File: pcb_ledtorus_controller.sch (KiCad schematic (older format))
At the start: 27 parts, among them P7 CONN_4X2, P8 CONN_9, U1 TM4C1232XXPM, U3 KNUSB, X1 NX5032GA-16MHz

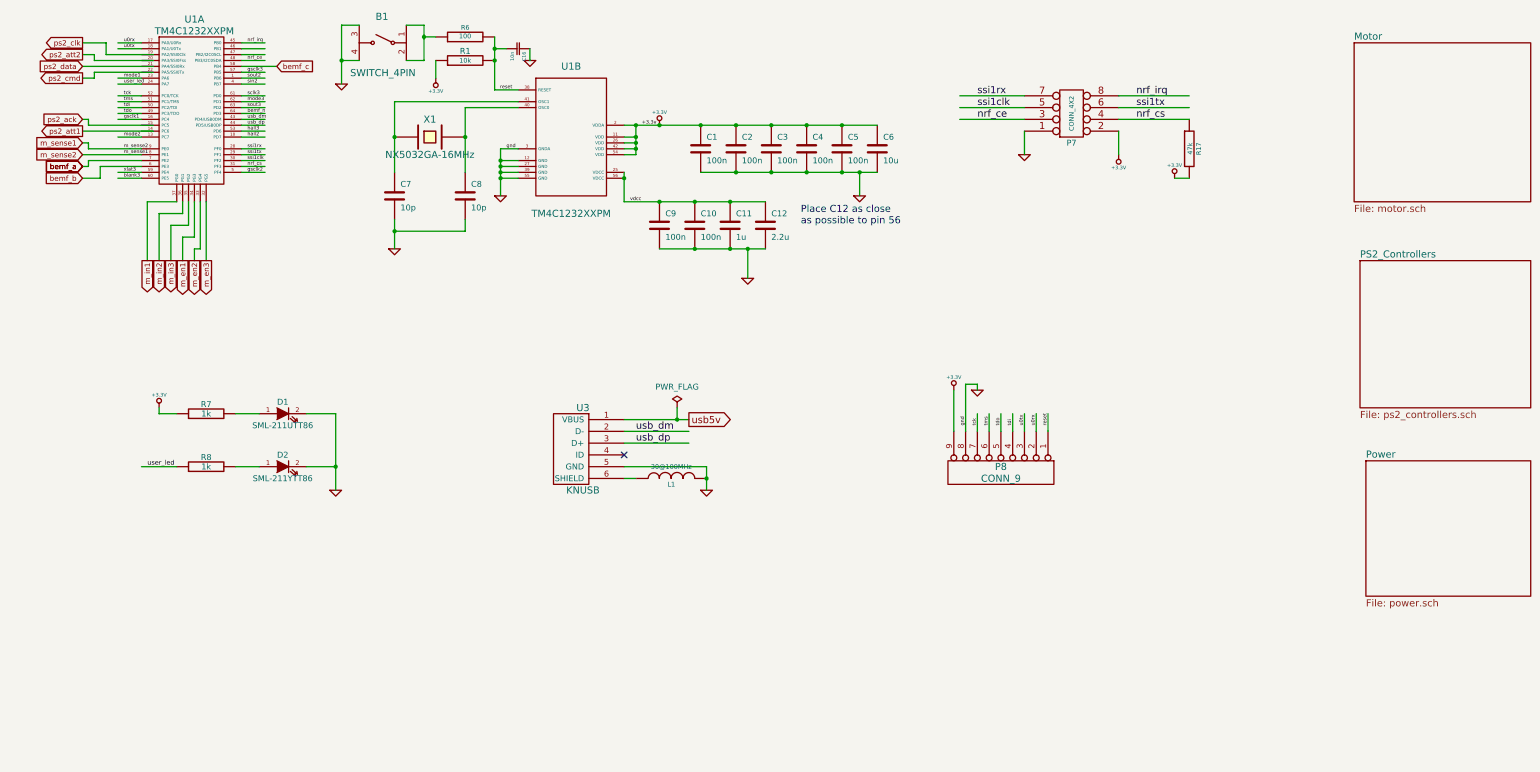
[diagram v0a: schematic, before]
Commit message: Passing ERC
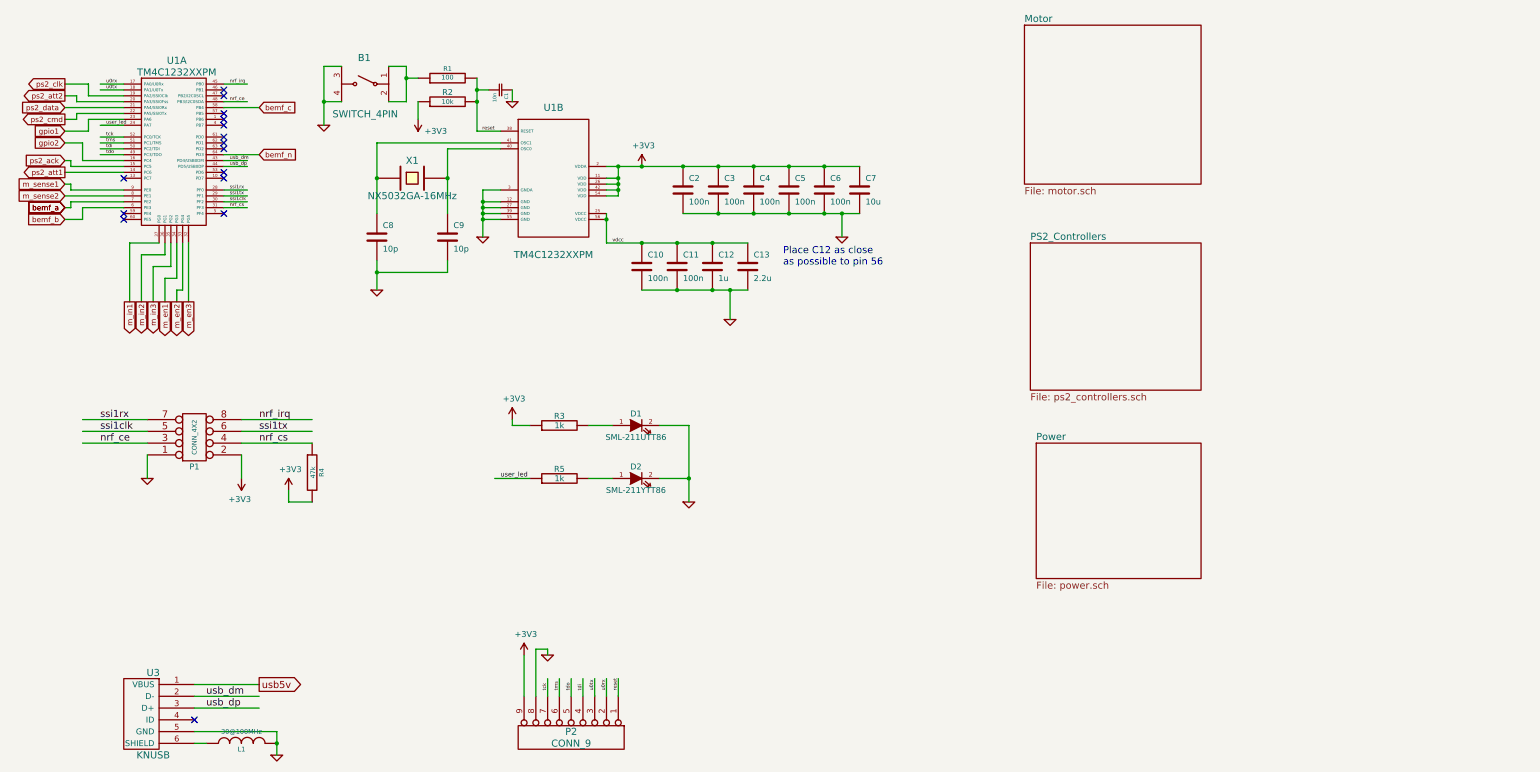
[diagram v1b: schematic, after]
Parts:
- renumbered C16 to C1, C9 to C10, C10 to C11, C11 to C12, C12 to C13, C1 to C2, C2 to C3, C3 to C4, C4 to C5, C5 to C6, C6 to C7, C7 to C8, C8 to C9, P7 to P1, P8 to P2, R6 to R1, R1 to R2, R7 to R3, R17 to R4, R8 to R5
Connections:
- net labels added: +3V3, gpio1, gpio2
- net labels removed: +3.3V, +3.3v, blank3, gnd, gsclk1, gsclk2, gsclk3, hall2, hall3, mode1, mode2, mode3, sclk3, sin2, sout2, sout3, xlat3
- wire segments 144 -> 134
- no-connect marks 1 -> 15
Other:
- moved on the sheet: B1, C1, C10, C11, C12, C13, C2, C3, C4, C5, C6, C7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

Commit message: Starting on netlist
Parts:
- B1: footprint (none) -> knielsenlib:SWITCH_FSMJSMA
- C1, C12, C13, C7, C8, C9: footprint (none) -> Capacitors_SMD:C_0805
- C10, C11, C2, C3, C4, C5, C6: footprint (none) -> Capacitors_SMD:C_0603
- D1, D2: footprint (none) -> LEDs:LED_0805
- L1: footprint (none) -> Inductors_SMD:L_0603
- P1: footprint (none) -> Pin_Headers:Pin_Header_Straight_2x04_Pitch1.27mm
- P2: footprint (none) -> Pin_Headers:Pin_Header_Straight_1x09_Pitch1.27mm
- R1, R2, R3, R4, R5: footprint (none) -> Resistors_SMD:R_0805
- U1: footprint (none) -> knielsenlib:LQFP_64
- U3: footprint (none) -> knielsenlib:10103594-0001LF
- X1: footprint (none) -> knielsenlib:NX5032GA
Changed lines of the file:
@@
 LIBS:w_device
 LIBS:pcb_ledtorus_controller-cache
-LIBS:tiva_pcb1-cache
 EELAYER 26 0
 EELAYER END
@@
 F 0 "R2" V 4630 1550 50  0000 C CNN
 F 1 "10k" V 4550 1550 40  0000 C CNN
-F 2 "" H 4550 1550 60  0001 C CNN
+F 2 "Resistors_SMD:R_0805" H 4550 1550 60  0001 C CNN
 F 3 "" H 4550 1550 60  0001 C CNN
 	1    4550 1550
@@
 F 0 "C7" H 8100 2400 50  0000 L CNN
 F 1 "10u" H 8100 2200 50  0000 L CNN
-F 2 "" H 8050 2300 60  0001 C CNN
+F 2 "Capacitors_SMD:C_0805" H 8050 2300 60  0001 C CNN
 F 3 "" H 8050 2300 60  0001 C CNN
 	1    8050 2300
@@
 F 0 "C6" H 7800 2400 50  0000 L CNN
 F 1 "100n" H 7800 2200 50  0000 L CNN
-F 2 "" H 7750 2300 60  0001 C CNN
+F 2 "Capacitors_SMD:C_0603" H 7750 2300 60  0001 C CNN
 F 3 "" H 7750 2300 60  0001 C CNN
 	1    7750 2300
@@
 F 0 "C2" H 6600 2400 50  0000 L CNN
 F 1 "100n" H 6600 2200 50  0000 L CNN
-F 2 "" H 6550 2300 60  0001 C CNN
+F 2 "Capacitors_SMD:C_0603" H 6550 2300 60  0001 C CNN
 F 3 "" H 6550 2300 60  0001 C CNN
 	1    6550 2300
@@
 F 0 "C3" H 6900 2400 50  0000 L CNN
 F 1 "100n" H 6900 2200 50  0000 L CNN
-F 2 "" H 6850 2300 60  0001 C CNN
+F 2 "Capacitors_SMD:C_0603" H 6850 2300 60  0001 C CNN
 F 3 "" H 6850 2300 60  0001 C CNN
 	1    6850 2300
@@
 F 0 "C4" H 7200 2400 50  0000 L CNN
 F 1 "100n" H 7200 2200 50  0000 L CNN
-F 2 "" H 7150 2300 60  0001 C CNN
+F 2 "Capacitors_SMD:C_0603" H 7150 2300 60  0001 C CNN
 F 3 "" H 7150 2300 60  0001 C CNN
 	1    7150 2300
@@
 F 0 "C5" H 7500 2400 50  0000 L CNN
 F 1 "100n" H 7500 2200 50  0000 L CNN
-F 2 "" H 7450 2300 60  0001 C CNN
+F 2 "Capacitors_SMD:C_0603" H 7450 2300 60  0001 C CNN
 F 3 "" H 7450 2300 60  0001 C CNN
 	1    7450 2300
@@
 F 0 "C13" H 7150 3050 50  0000 L CNN
 F 1 "2.2u" H 7150 2850 50  0000 L CNN
-F 2 "" H 7100 2950 60  0001 C CNN
+F 2 "Capacitors_SMD:C_0805" H 7100 2950 60  0001 C CNN
 F 3 "" H 7100 2950 60  0001 C CNN
 	1    7100 2950
@@
 F 0 "C12" H 6850 3050 50  0000 L CNN
 F 1 "1u" H 6850 2850 50  0000 L CNN
-F 2 "" H 6800 2950 60  0001 C CNN
+F 2 "Capacitors_SMD:C_0805" H 6800 2950 60  0001 C CNN
 F 3 "" H 6800 2950 60  0001 C CNN
 	1    6800 2950
@@
 F 0 "C11" H 6550 3050 50  0000 L CNN
 F 1 "100n" H 6550 2850 50  0000 L CNN
-F 2 "" H 6500 2950 60  0001 C CNN
+F 2 "Capacitors_SMD:C_0603" H 6500 2950 60  0001 C CNN
 F 3 "" H 6500 2950 60  0001 C CNN
 	1    6500 2950
@@
 F 0 "C10" H 6250 3050 50  0000 L CNN
 F 1 "100n" H 6250 2850 50  0000 L CNN
-F 2 "" H 6200 2950 60  0001 C CNN
+F 2 "Capacitors_SMD:C_0603" H 6200 2950 60  0001 C CNN
 F 3 "" H 6200 2950 60  0001 C CNN
 	1    6200 2950
@@
 F 0 "C9" H 4600 2800 50  0000 L CNN
 F 1 "10p" H 4600 2600 50  0000 L CNN
-F 2 "" H 4550 2700 60  0001 C CNN
+F 2 "Capacitors_SMD:C_0805" H 4550 2700 60  0001 C CNN
 F 3 "" H 4550 2700 60  0001 C CNN
 	1    4550 2700
@@
 F 0 "C8" H 4000 2800 50  0000 L CNN
 F 1 "10p" H 4000 2600 50  0000 L CNN
-F 2 "" H 3950 2700 60  0001 C CNN
+F 2 "Capacitors_SMD:C_0805" H 3950 2700 60  0001 C CNN
 F 3 "" H 3950 2700 60  0001 C CNN
 	1    3950 2700
@@
 F 0 "X1" H 4250 2350 60  0000 C CNN
 F 1 "NX5032GA-16MHz" H 4250 2050 60  0000 C CNN
-F 2 "" H 4250 2200 60  0001 C CNN
+F 2 "knielsenlib:NX5032GA" H 4250 2200 60  0001 C CNN
 F 3 "" H 4250 2200 60  0001 C CNN
 	1    4250 2200
@@
 F 0 "U1" H 5450 2700 60  0000 C CNN
 F 1 "TM4C1232XXPM" H 5450 1450 60  0000 C CNN
-F 2 "" H 5450 2150 60  0001 C CNN
+F 2 "knielsenlib:LQFP_64" H 5450 2150 60  0001 C CNN
 F 3 "" H 5450 2150 60  0001 C CNN
 	2    5450 2150
@@
 F 0 "U1" H 2250 2800 60  0000 C CNN
 F 1 "TM4C1232XXPM" H 2250 2700 60  0000 C CNN
-F 2 "" H 2250 2000 60  0000 C CNN
+F 2 "knielsenlib:LQFP_64" H 2250 2000 60  0001 C CNN
 F 3 "" H 2250 2000 60  0000 C CNN
 	1    2250 2000
@@
 F 0 "U3" H 2050 6400 60  0000 C CNN
 F 1 "KNUSB" H 2050 5700 60  0000 C CNN
-F 2 "" H 2050 6400 60  0000 C CNN
+F 2 "knielsenlib:10103594-0001LF" H 2050 6400 60  0001 C CNN
 F 3 "" H 2050 6400 60  0000 C CNN
 	1    2050 6400
@@
 F 0 "L1" V 2750 7000 40  0000 C CNN
 F 1 "30@100MHz" V 2900 7000 40  0000 C CNN
-F 2 "" H 2800 7000 60  0000 C CNN
+F 2 "Inductors_SMD:L_0603" H 2800 7000 60  0001 C CNN
 F 3 "" H 2800 7000 60  0000 C CNN
 	1    2800 7000
@@
 F 0 "B1" H 3857 1623 60  0000 C CNN
 F 1 "SWITCH_4PIN" H 3849 1145 60  0000 C CNN
-F 2 "" H 3850 1400 60  0000 C CNN
+F 2 "knielsenlib:SWITCH_FSMJSMA" H 3850 1400 60  0001 C CNN
 F 3 "" H 3850 1400 60  0000 C CNN
 	1    3850 1400
@@
 F 0 "R1" V 4630 1350 40  0000 C CNN
 F 1 "100" V 4557 1351 40  0000 C CNN
-F 2 "" V 4480 1350 30  0000 C CNN
+F 2 "Resistors_SMD:R_0805" V 4480 1350 30  0001 C CNN
 F 3 "" H 4550 1350 30  0000 C CNN
 	1    4550 1350
@@
 F 0 "C1" H 5025 1500 30  0000 L CNN
 F 1 "10n" H 5025 1400 30  0000 L CNN
-F 2 "" H 5000 1450 60  0000 C CNN
+F 2 "Capacitors_SMD:C_0805" H 5000 1450 60  0001 C CNN
 F 3 "" H 5000 1450 60  0000 C CNN
 	1    5000 1450
@@
 F 0 "R5" V 5580 4750 50  0000 C CNN
 F 1 "1k" V 5500 4750 50  0000 C CNN
-F 2 "" H 5500 4750 60  0001 C CNN
+F 2 "Resistors_SMD:R_0805" H 5500 4750 60  0001 C CNN
 F 3 "" H 5500 4750 60  0001 C CNN
 	1    5500 4750
@@
 F 0 "R3" V 5580 4300 50  0000 C CNN
 F 1 "1k" V 5500 4300 50  0000 C CNN
-F 2 "" H 5500 4300 60  0001 C CNN
+F 2 "Resistors_SMD:R_0805" H 5500 4300 60  0001 C CNN
 F 3 "" H 5500 4300 60  0001 C CNN
 	1    5500 4300
@@
 F 0 "D2" H 6150 4850 50  0000 C CNN
 F 1 "SML-211YTT86" H 6150 4650 50  0000 C CNN
-F 2 "" H 6150 4750 60  0001 C CNN
+F 2 "LEDs:LED_0805" H 6150 4750 60  0001 C CNN
 F 3 "" H 6150 4750 60  0001 C CNN
 	1    6150 4750
@@
 F 0 "D1" H 6150 4400 50  0000 C CNN
 F 1 "SML-211UTT86" H 6150 4200 50  0000 C CNN
-F 2 "" H 6150 4300 60  0001 C CNN
+F 2 "LEDs:LED_0805" H 6150 4300 60  0001 C CNN
 F 3 "" H 6150 4300 60  0001 C CNN
 	1    6150 4300
@@
 F 0 "P1" H 2400 4650 50  0000 C CNN
 F 1 "CONN_4X2" V 2400 4400 40  0000 C CNN
-F 2 "" H 2400 4400 60  0000 C CNN
+F 2 "Pin_Headers:Pin_Header_Straight_2x04_Pitch1.27mm" H 2400 4400 60  0001 C CNN
 F 3 "" H 2400 4400 60  0000 C CNN
 	1    2400 4400
@@
 F 0 "P2" V 5550 6950 60  0000 C CNN
 F 1 "CONN_9" V 5650 6950 60  0000 C CNN
-F 2 "" H 5600 6950 60  0000 C CNN
+F 2 "Pin_Headers:Pin_Header_Straight_1x09_Pitch1.27mm" H 5600 6950 60  0001 C CNN
 F 3 "" H 5600 6950 60  0000 C CNN
 	1    5600 6950
@@
 F 0 "R4" V 3480 4700 40  0000 C CNN
 F 1 "47k" V 3407 4701 40  0000 C CNN
-F 2 "" V 3330 4700 30  0000 C CNN
+F 2 "Resistors_SMD:R_0805" V 3330 4700 30  0001 C CNN
 F 3 "" H 3400 4700 30  0000 C CNN
 	1    3400 4700

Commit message: Starting on netlist
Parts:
- P1: footprint Pin_Headers:Pin_Header_Straight_2x04_Pitch1.27mm -> Pin_Headers:Pin_Header_Straight_2x04_Pitch2.54mm
- P2: footprint Pin_Headers:Pin_Header_Straight_1x09_Pitch1.27mm -> Pin_Headers:Pin_Header_Straight_1x09_Pitch2.54mm
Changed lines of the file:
@@
 LIBS:contrib
 LIBS:valves
-LIBS:w_analog
-LIBS:w_device
 LIBS:pcb_ledtorus_controller-cache
 EELAYER 26 0
@@
 F 0 "P1" H 2400 4650 50  0000 C CNN
 F 1 "CONN_4X2" V 2400 4400 40  0000 C CNN
-F 2 "Pin_Headers:Pin_Header_Straight_2x04_Pitch1.27mm" H 2400 4400 60  0001 C CNN
+F 2 "Pin_Headers:Pin_Header_Straight_2x04_Pitch2.54mm" H 2400 4400 60  0001 C CNN
 F 3 "" H 2400 4400 60  0000 C CNN
 	1    2400 4400
@@
 F 0 "P2" V 5550 6950 60  0000 C CNN
 F 1 "CONN_9" V 5650 6950 60  0000 C CNN
-F 2 "Pin_Headers:Pin_Header_Straight_1x09_Pitch1.27mm" H 5600 6950 60  0001 C CNN
+F 2 "Pin_Headers:Pin_Header_Straight_1x09_Pitch2.54mm" H 5600 6950 60  0001 C CNN
 F 3 "" H 5600 6950 60  0000 C CNN
 	1    5600 6950

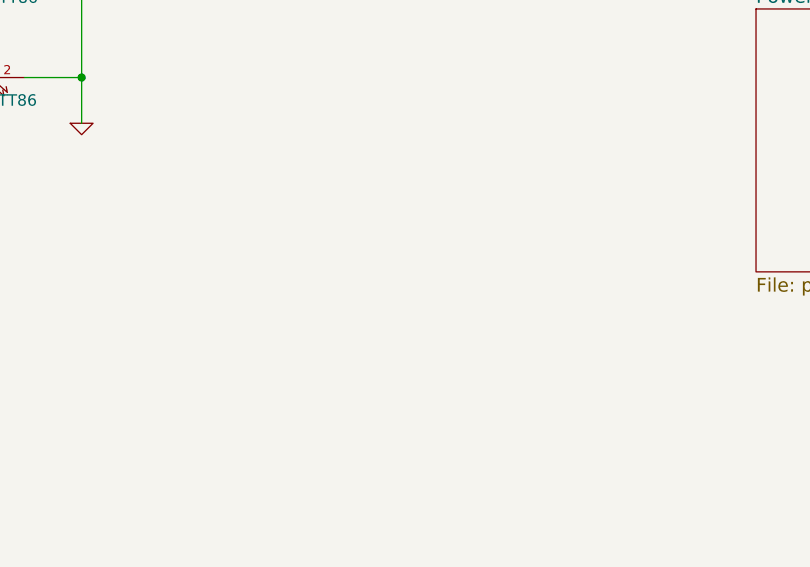
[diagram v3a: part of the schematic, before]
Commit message: Work on layout
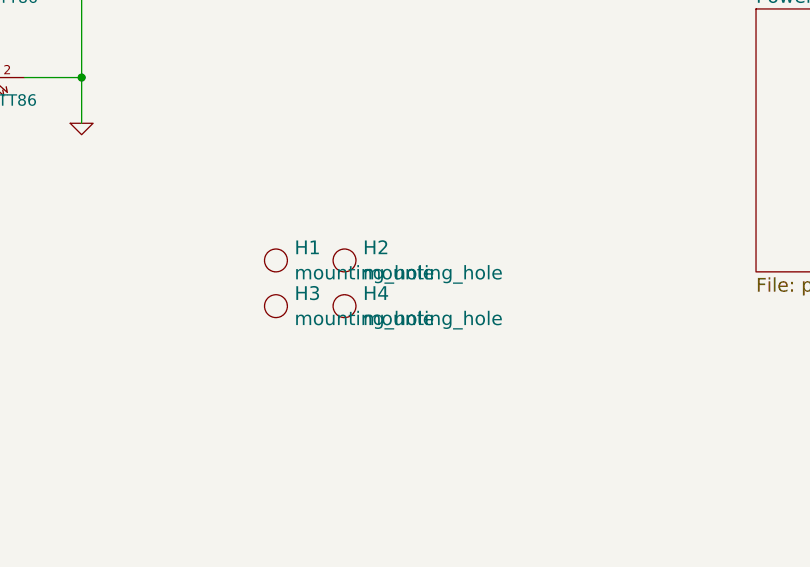
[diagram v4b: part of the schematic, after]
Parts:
- added H1, H2, H3, H4: mounting_hole, Mounting_Holes:MountingHole_4.3mm_M4, symbol mounting_hole
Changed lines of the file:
@@
 	-1   0    0    1
 $EndComp
+$Comp
+L mounting_hole H1
+U 1 1 5C292E61
+P 7450 5550
+F 0 "H1" H 7531 5605 60  0000 L CNN
+F 1 "mounting_hole" H 7531 5495 60  0000 L CNN
+F 2 "Mounting_Holes:MountingHole_4.3mm_M4" H 7450 5550 60  0001 C CNN
+F 3 "" H 7450 5550 60  0000 C CNN
+	1    7450 5550
+	1    0    0    -1
+$EndComp
+$Comp
+L mounting_hole H3
+U 1 1 5C292F44
+P 7450 5750
+F 0 "H3" H 7531 5805 60  0000 L CNN
+F 1 "mounting_hole" H 7531 5695 60  0000 L CNN
+F 2 "Mounting_Holes:MountingHole_4.3mm_M4" H 7450 5750 60  0001 C CNN
+F 3 "" H 7450 5750 60  0000 C CNN
+	1    7450 5750
+	1    0    0    -1
+$EndComp
+$Comp
+L mounting_hole H2
+U 1 1 5C292F9F
+P 7750 5550
+F 0 "H2" H 7831 5605 60  0000 L CNN
+F 1 "mounting_hole" H 7831 5495 60  0000 L CNN
+F 2 "Mounting_Holes:MountingHole_4.3mm_M4" H 7750 5550 60  0001 C CNN
+F 3 "" H 7750 5550 60  0000 C CNN
+	1    7750 5550
+	1    0    0    -1
+$EndComp
+$Comp
+L mounting_hole H4
+U 1 1 5C293020
+P 7750 5750
+F 0 "H4" H 7831 5805 60  0000 L CNN
+F 1 "mounting_hole" H 7831 5695 60  0000 L CNN
+F 2 "Mounting_Holes:MountingHole_4.3mm_M4" H 7750 5750 60  0001 C CNN
+F 3 "" H 7750 5750 60  0000 C CNN
+	1    7750 5750
+	1    0    0    -1
+$EndComp
 $EndSCHEMATC
